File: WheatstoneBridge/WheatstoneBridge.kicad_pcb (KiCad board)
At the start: 2 copper layers, 100 x 50 mm, 6 parts

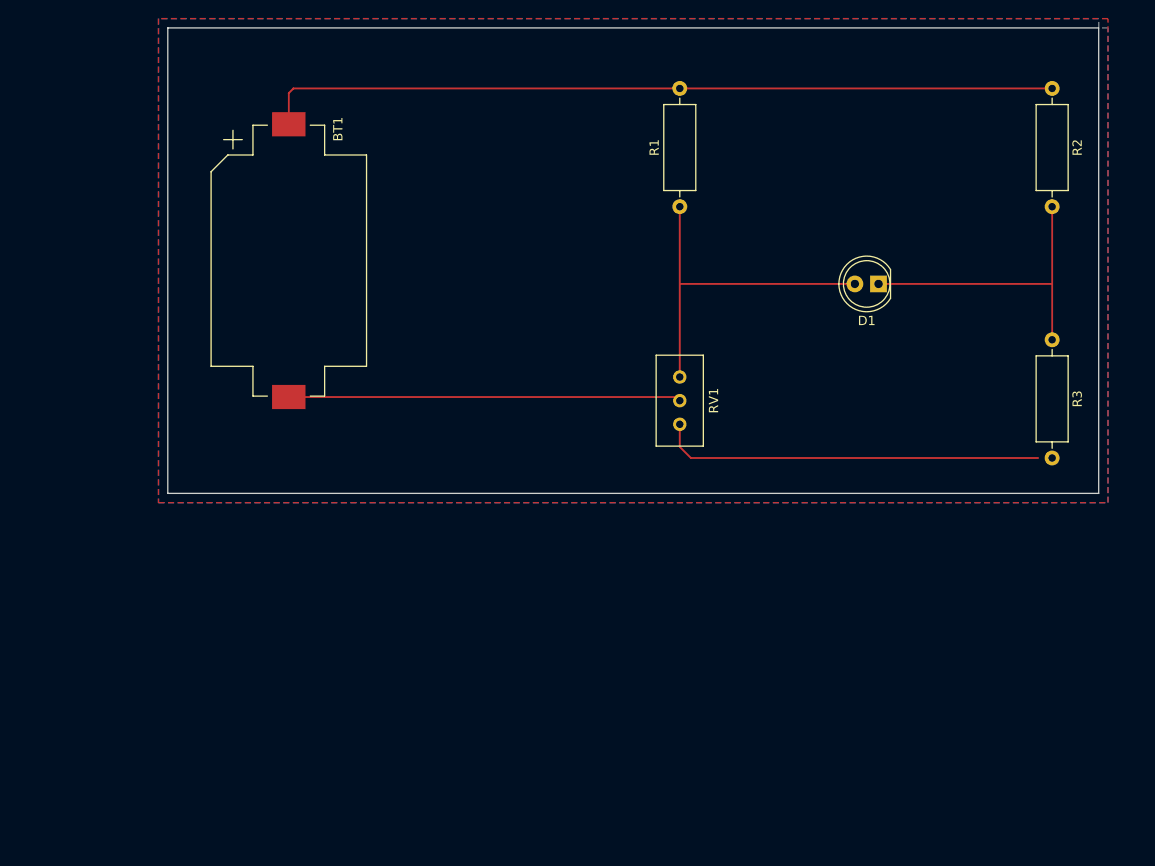
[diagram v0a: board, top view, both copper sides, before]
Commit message: Update wheatstonebridges
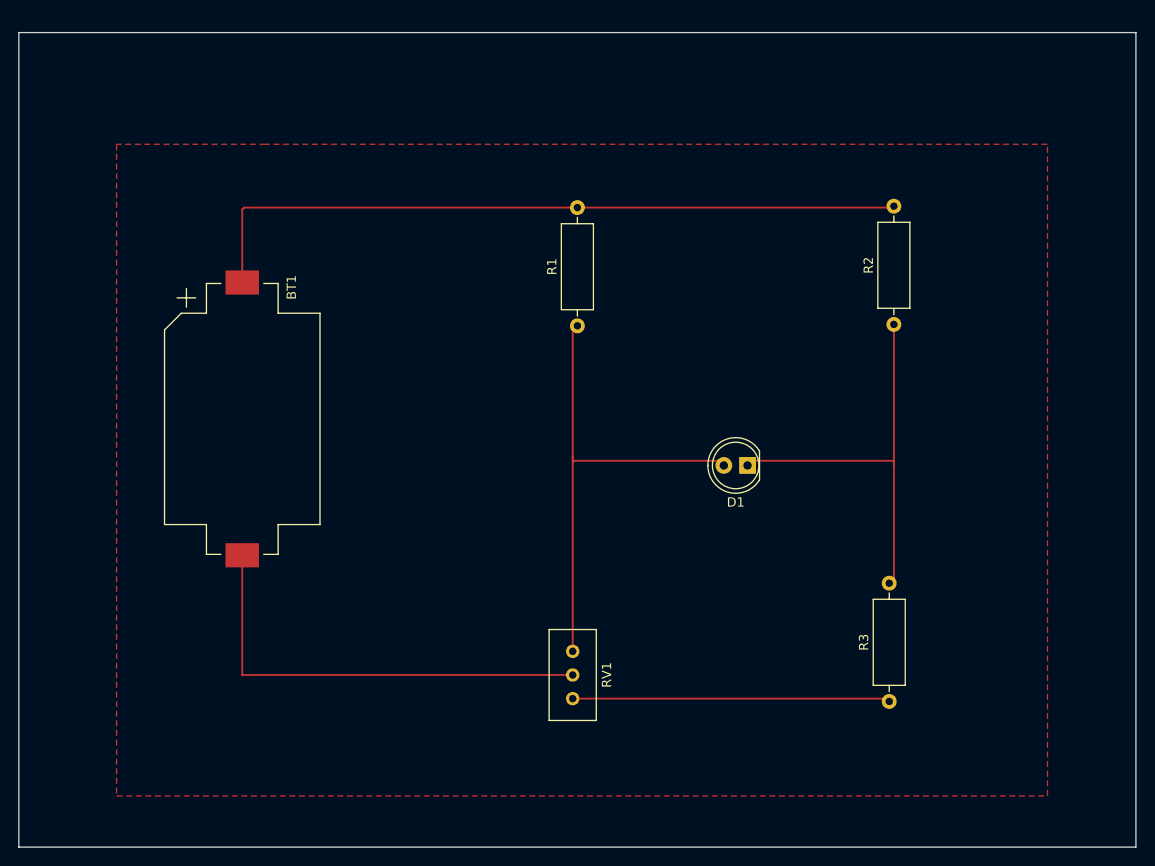
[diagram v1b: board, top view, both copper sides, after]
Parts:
- BT1: value 10V -> 10
- D1: value red -> LED
- R1: value 0.5k -> 500
- R3: value 0.15k -> 150
- moved R3 42.6 mm to (177.5, 122.3), turned to 90 degrees
- moved RV1 31.6 mm to (143.5, 122.0)
- moved R2 30.5 mm to (178.0, 81.8), turned to 90 degrees
- moved D1 24.0 mm to (162.3, 97.0)
- moved BT1 17.7 mm to (108.0, 92.0)
- moved R1 16.9 mm to (144.0, 82.0)
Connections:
- R2 pad 1: VCC -> Net-(D1-K)
- R2 pad 2: Net-(D1-K) -> VCC
- R3 pad 1: Net-(D1-K) -> GND
- R3 pad 2: GND -> Net-(D1-K)
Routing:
- net Net-(D1-A): track 37.1 -> 52.4 mm
- net Net-(D1-K): track 33.0 -> 44.4 mm
- net VCC: track 85.6 -> 78.0 mm
- net GND: track 83.6 -> 82.5 mm
- removed copper zone on B.Cu, net GND
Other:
- board size 100 x 50 mm -> 120 x 87.5 mm
